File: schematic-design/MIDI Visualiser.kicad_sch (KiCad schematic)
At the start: 21 parts, among them J1 POWER Barrel Jack, J2 DIN-5_180degree, J3 DIN-5_180degree, J4 Conn_01x03_Pin, U1 6N138 Optocoupler, U1 ATmega328P-P, U2 LM2574Y-5 Buck converter, U3 74LS04, Y1 Crystal

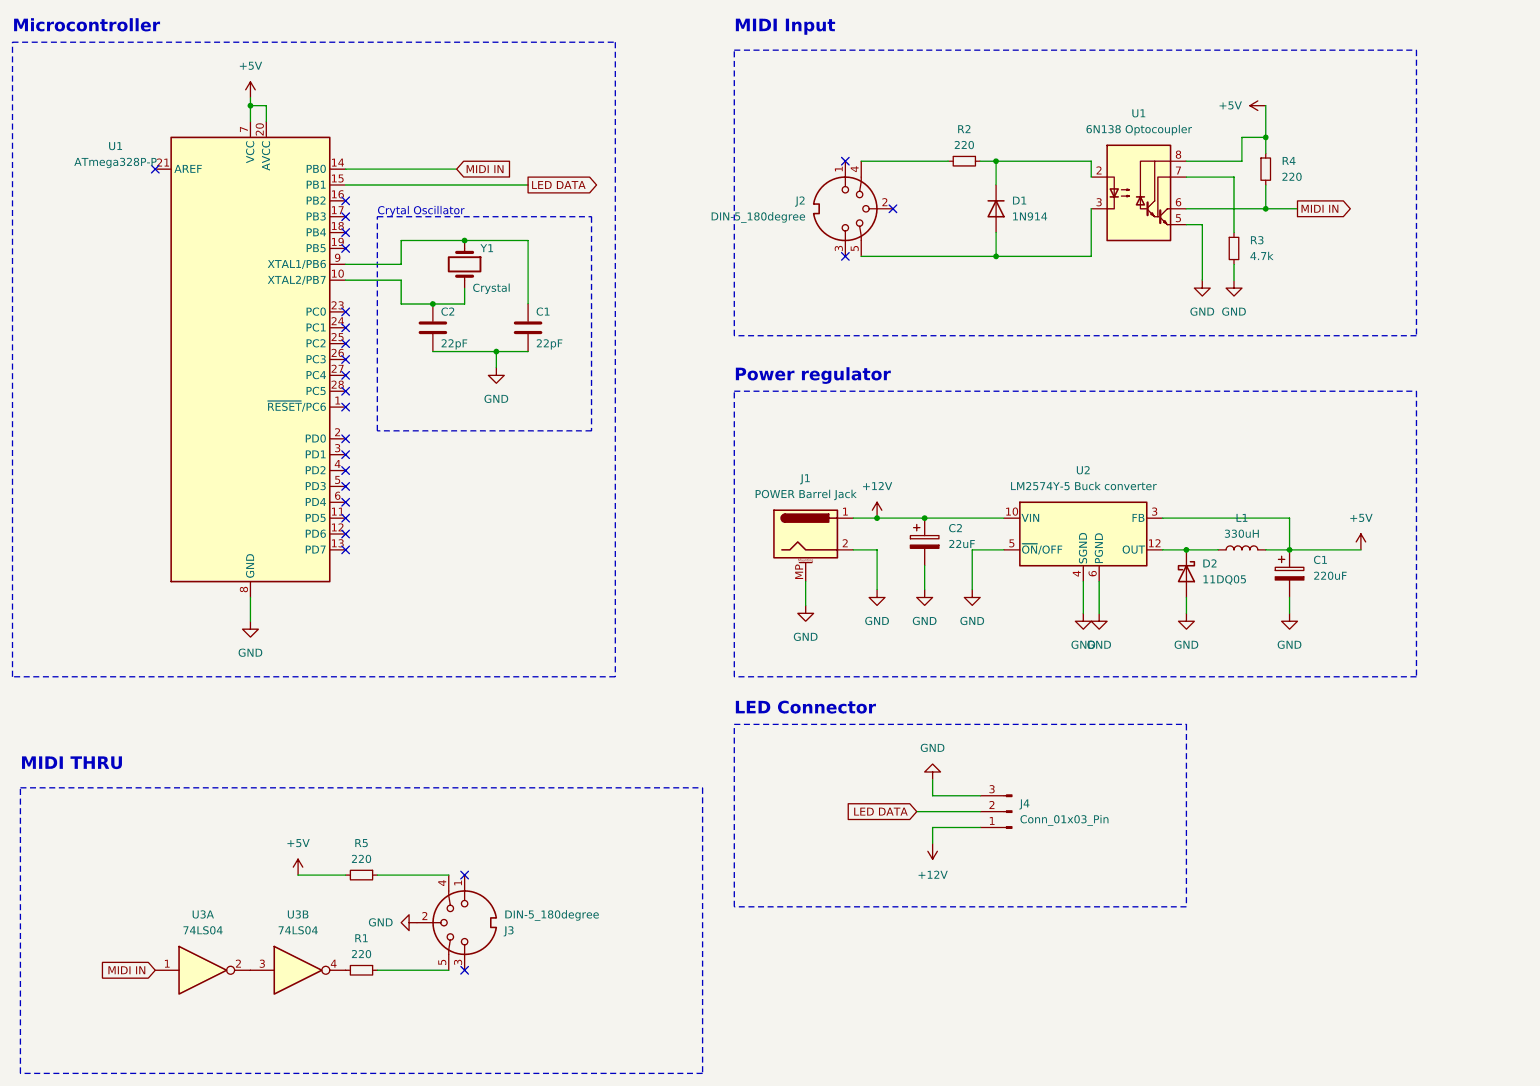
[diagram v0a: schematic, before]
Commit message: Replace MIDI Visualiser.kicad_sch
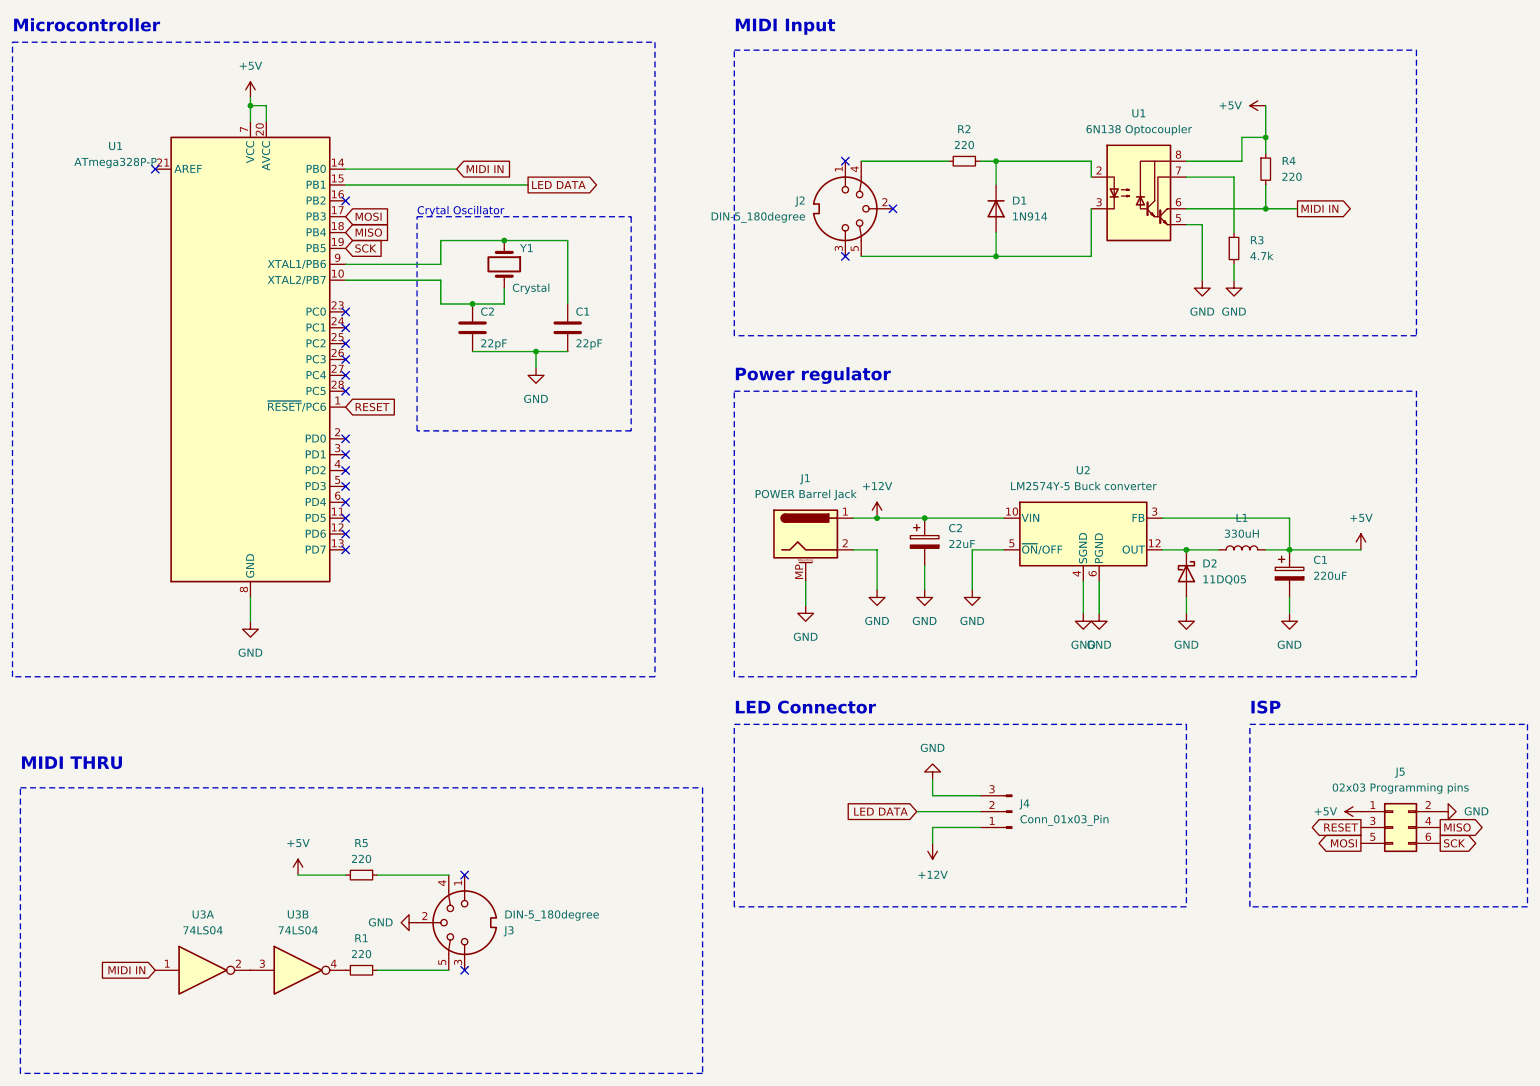
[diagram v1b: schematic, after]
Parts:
- added J5: 02x03 Programming pins, symbol Connector_Generic:Conn_02x03_Odd_Even
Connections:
- net +5V: now also J5.1 (Pin_1)
- net GND: now also J5.2 (Pin_2)
- net RESET: now reaches U1.1 (~{RESET}/PC6)
- net RESET: now also J5.3 (Pin_3)
- net MOSI: now reaches U1.17 (PB3)
- net MOSI: now also J5.5 (Pin_5)
- net MISO: now reaches U1.18 (PB4)
- net MISO: now also J5.4 (Pin_4)
- net SCK: now reaches U1.19 (PB5)
- net SCK: now also J5.6 (Pin_6)
- no-connect marks 25 -> 21
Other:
- note added: "ISP"
- moved on the sheet: C1, C2, Y1
